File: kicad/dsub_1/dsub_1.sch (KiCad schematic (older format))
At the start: 3 parts, among them J1 DB15_Female, J2 DB15_Female, J3 DB25_Female

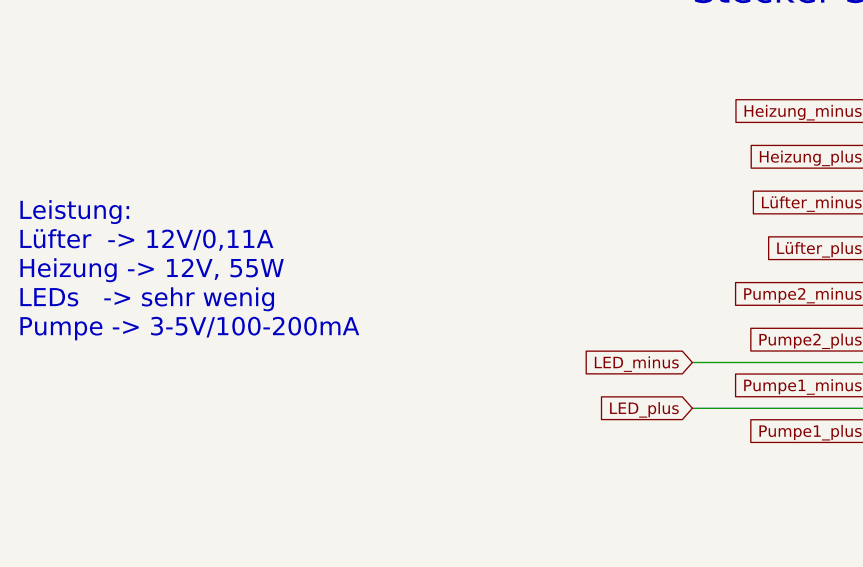
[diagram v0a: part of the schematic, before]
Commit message: geändert:       Doku/Anmerungen_fuer_Doku.odt 	geändert:       Doku/Tagebuch_Ziele.odt 	geändert:       abschlussprojekt/abschlussprojekt.ino -> Helligkeitssensor + LEDs implementiert 	geändert:       kicad/dsub_1/dsub_1.bak 	geändert:       kicad/dsub_1/dsub_1.pdf 	geändert:       kicad/dsub_1/dsub_1.sch
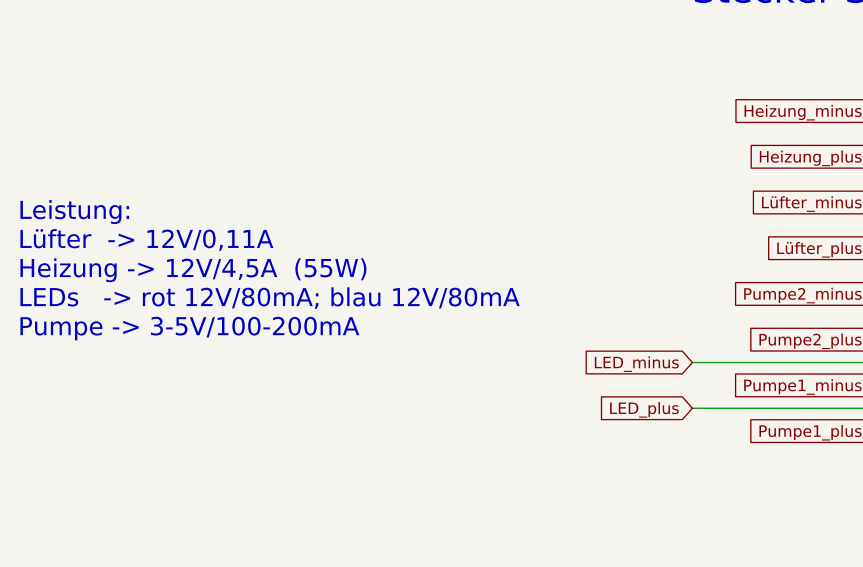
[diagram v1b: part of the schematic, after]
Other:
- note added: "Leistung:\nLüfter -> 12V/0,11A\nHeizung -> 12V/4,5A (55W)\nLEDs -> rot 12V/80mA; blau 12V/80mA\nPumpe -> 3-5V/100-200mA\n"
- note removed: "Leistung:\nLüfter -> 12V/0,11A\nHeizung -> 12V, 55W\nLEDs -> sehr wenig\nPumpe -> 3-5V/100-200mA\n"
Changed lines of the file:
@@
 Stecker:\nTorsten -> Männchen, Male\nFabian -> Weibchen, Female
 Text Notes 700  5250 0    79   ~ 0
-Leistung:\nLüfter  -> 12V/0,11A\nHeizung -> 12V, 55W\nLEDs   -> sehr wenig\nPumpe -> 3-5V/100-200mA\n
+Leistung:\nLüfter  -> 12V/0,11A\nHeizung -> 12V/4,5A  (55W)\nLEDs   -> rot 12V/80mA; blau 12V/80mA\nPumpe -> 3-5V/100-200mA\n
 $Comp
 L Connector:DB15_Female J2
